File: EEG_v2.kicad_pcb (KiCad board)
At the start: 2 copper layers, 114 parts, among them P1 CONN_2, P2 CONN_8, P3 USB_A, P4 CONN_8, P5 CONN_5X2, P6 CONN_2, P7 CONN_1, SW1 SWITCH_INV, SW2 RESET, SW3 SW_PUSH_4PIN, SW4 SW_PUSH_4PIN, U1 ADS1299IPAGR, U2 TLV70033, U3 TLV70025, U4 LM2664, U5 TPS72325, U6 CC2540, U7 2450BM15A0002E, X1 QUARTZCMS4_32K, X2 32-MHz

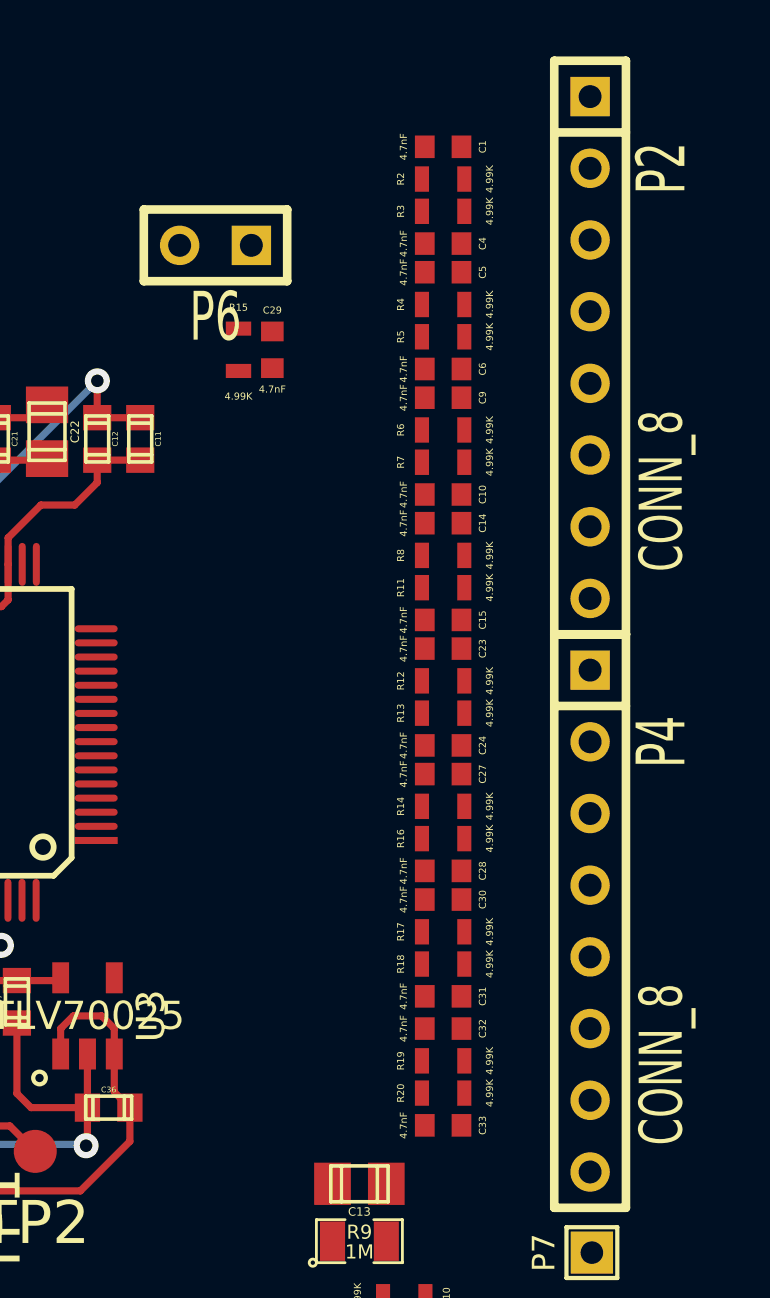
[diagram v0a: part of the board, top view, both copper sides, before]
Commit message: Continue layout.
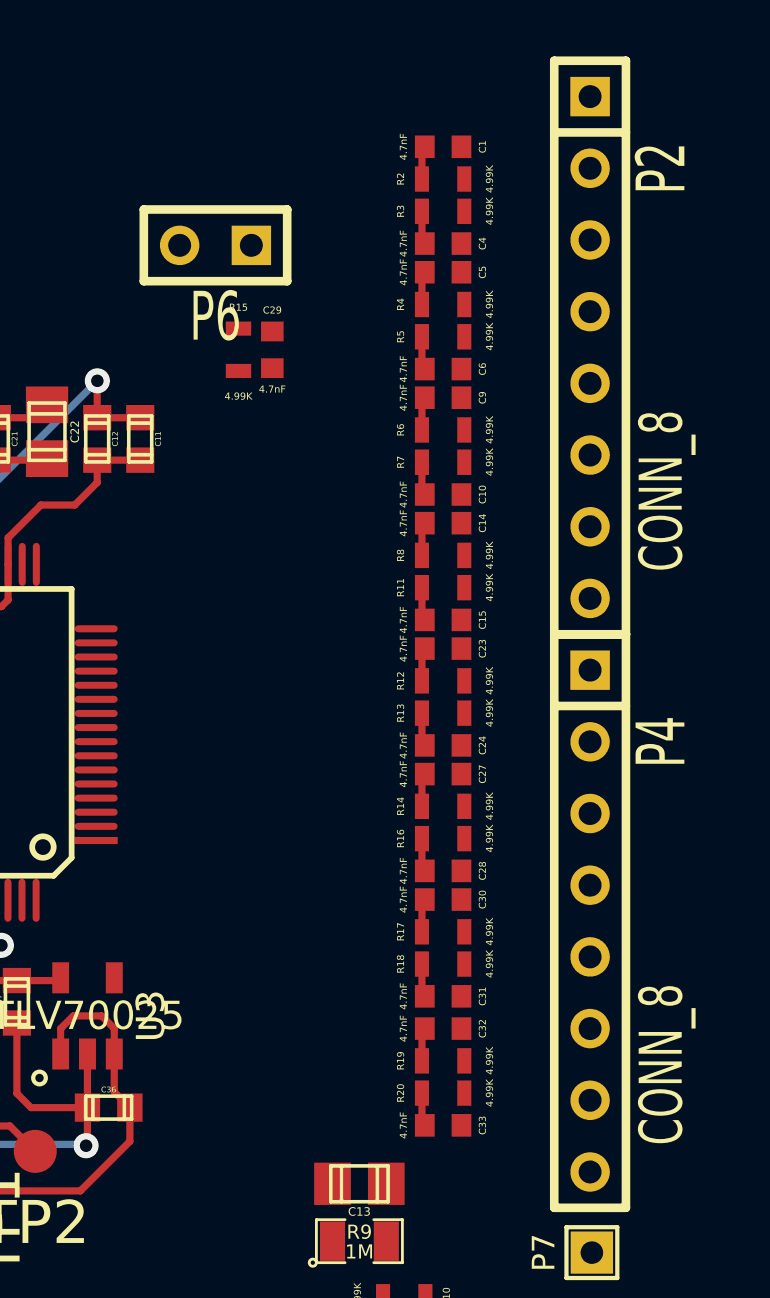
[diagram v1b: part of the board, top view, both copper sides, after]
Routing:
- net N-0000096: track 0.00 -> 1.18 mm
- net N-0000094: track 0.00 -> 1.18 mm
- net N-0000093: track 0.00 -> 1.18 mm
- net N-0000092: track 0.00 -> 1.18 mm
- net N-0000091: track 0.00 -> 1.18 mm
- net N-0000090: track 0.00 -> 1.18 mm
- net N-0000089: track 0.00 -> 1.18 mm
- net N-0000088: track 0.00 -> 1.18 mm
- net N-0000078: track 0.00 -> 1.18 mm
- net N-0000077: track 0.00 -> 1.18 mm
- net N-0000076: track 0.00 -> 1.18 mm
- net N-0000070: track 0.00 -> 1.18 mm
- net N-0000067: track 0.00 -> 1.18 mm
- net N-0000095: track 0.00 -> 1.18 mm
- net N-0000079: track 0.00 -> 1.18 mm
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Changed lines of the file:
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@@
   (general
     (links 295)
-    (no_connects 193)
+    (no_connects 177)
     (area 249.516999 132.753099 336.86877 191.129001)
     (thickness 1.6)
-    (drawings 0)
-    (tracks 263)
+    (drawings 1)
+    (tracks 295)
     (zones 0)
     (modules 114)
@@
     )
   )
+  (dimension 43.501839 (width 0.3) (layer F.SilkS)
+    (gr_text "43.502 mm" (at 345.328961 154.844059 89.47315711) (layer F.SilkS)
+      (effects (font (size 1.5 1.5) (thickness 0.3)))
+    )
+    (feature1 (pts (xy 334.9 176.5) (xy 346.478904 176.606472)))
+    (feature2 (pts (xy 335.3 133) (xy 346.878904 133.106472)))
+    (crossbar (pts (xy 344.179019 133.081646) (xy 343.779019 176.581646)))
+    (arrow1a (pts (xy 343.779019 176.581646) (xy 343.202982 175.449798)))
+    (arrow1b (pts (xy 343.779019 176.581646) (xy 344.375773 175.460583)))
+    (arrow2a (pts (xy 344.179019 133.081646) (xy 343.582265 134.202709)))
+    (arrow2b (pts (xy 344.179019 133.081646) (xy 344.755056 134.213494)))
+  )
   (segment (start 311.85184 165.74816) (end 311.85184 165.35184) (width 0.254) (layer F.Cu) (net 1))
   (segment (start 310.93156 164.43156) (end 310.93156 162.90544) (width 0.254) (layer F.Cu) (net 1))
@@
   (segment (start 305.27116 172.67884) (end 305.27116 170.58) (width 0.254) (layer F.Cu) (net 59))
   (segment (start 304.957 172.993) (end 305.27116 172.67884) (width 0.254) (layer F.Cu) (net 59))
+  (segment (start 327.1005 142.9385) (end 327.1005 143.9815) (width 0.254) (layer F.Cu) (net 66) (status C00000))
+  (segment (start 327.1005 143.9815) (end 327.2005 144.0815) (width 0.254) (layer F.Cu) (net 66) (status C00000))
+  (segment (start 327.1005 137.3505) (end 327.1005 136.3075) (width 0.254) (layer F.Cu) (net 67) (status C00000))
+  (segment (start 327.1005 136.3075) (end 327.2005 136.2075) (width 0.254) (layer F.Cu) (net 67) (status C00000))
+  (segment (start 327.1005 138.4935) (end 327.1005 139.5365) (width 0.254) (layer F.Cu) (net 68) (status C00000))
+  (segment (start 327.1005 139.5365) (end 327.2005 139.6365) (width 0.254) (layer F.Cu) (net 68) (status C00000))
+  (segment (start 327.1005 147.3835) (end 327.1005 148.4265) (width 0.254) (layer F.Cu) (net 69) (status C00000))
+  (segment (start 327.1005 148.4265) (end 327.2005 148.5265) (width 0.254) (layer F.Cu) (net 69) (status C00000))
+  (segment (start 327.1005 141.7955) (end 327.1005 140.7525) (width 0.254) (layer F.Cu) (net 70) (status C00000))
+  (segment (start 327.1005 140.7525) (end 327.2005 140.6525) (width 0.254) (layer F.Cu) (net 70) (status C00000))
+  (segment (start 327.1005 146.2405) (end 327.1005 145.1975) (width 0.254) (layer F.Cu) (net 71) (status C00000))
+  (segment (start 327.1005 145.1975) (end 327.2005 145.0975) (width 0.254) (layer F.Cu) (net 71) (status C00000))
+  (segment (start 327.1005 150.6855) (end 327.1005 149.6425) (width 0.254) (layer F.Cu) (net 72) (status C00000))
+  (segment (start 327.1005 149.6425) (end 327.2005 149.5425) (width 0.254) (layer F.Cu) (net 72) (status C00000))
+  (segment (start 327.1005 169.7355) (end 327.1005 170.7785) (width 0.254) (layer F.Cu) (net 74) (status C00000))
+  (segment (start 327.1005 170.7785) (end 327.2005 170.8785) (width 0.254) (layer F.Cu) (net 74) (status C00000))
+  (segment (start 327.1005 168.5925) (end 327.1005 167.5495) (width 0.254) (layer F.Cu) (net 75) (status C00000))
+  (segment (start 327.1005 167.5495) (end 327.2005 167.4495) (width 0.254) (layer F.Cu) (net 75) (status C00000))
+  (segment (start 327.1005 159.5755) (end 327.1005 158.5325) (width 0.254) (layer F.Cu) (net 76) (status C00000))
+  (segment (start 327.1005 158.5325) (end 327.2005 158.4325) (width 0.254) (layer F.Cu) (net 76) (status C00000))
+  (segment (start 327.1005 160.7185) (end 327.1005 161.7615) (width 0.254) (layer F.Cu) (net 77) (status C00000))
+  (segment (start 327.1005 161.7615) (end 327.2005 161.8615) (width 0.254) (layer F.Cu) (net 77) (status C00000))
+  (segment (start 327.1005 164.0205) (end 327.1005 162.9775) (width 0.254) (layer F.Cu) (net 78) (status C00000))
+  (segment (start 327.1005 162.9775) (end 327.2005 162.8775) (width 0.254) (layer F.Cu) (net 78) (status C00000))
+  (segment (start 327.1005 165.1635) (end 327.1005 166.2065) (width 0.254) (layer F.Cu) (net 79) (status C00000))
+  (segment (start 327.1005 166.2065) (end 327.2005 166.3065) (width 0.254) (layer F.Cu) (net 79) (status C00000))
+  (segment (start 327.1005 151.8285) (end 327.1005 152.8715) (width 0.254) (layer F.Cu) (net 80) (status C00000))
+  (segment (start 327.1005 152.8715) (end 327.2005 152.9715) (width 0.254) (layer F.Cu) (net 80) (status C00000))
+  (segment (start 327.1005 156.2735) (end 327.1005 157.3165) (width 0.254) (layer F.Cu) (net 81) (status C00000))
+  (segment (start 327.1005 157.3165) (end 327.2005 157.4165) (width 0.254) (layer F.Cu) (net 81) (status C00000))
+  (segment (start 327.1005 155.1305) (end 327.1005 154.0875) (width 0.254) (layer F.Cu) (net 82) (status C00000))
+  (segment (start 327.1005 154.0875) (end 327.2005 153.9875) (width 0.254) (layer F.Cu) (net 82) (status C00000))
   (segment (start 292.9415 144.5455) (end 291.252 144.5455) (width 0.254) (layer F.Cu) (net 83))
   (segment (start 291.252 144.5455) (end 290.75 145.0475) (width 0.254) (layer F.Cu) (net 83))
